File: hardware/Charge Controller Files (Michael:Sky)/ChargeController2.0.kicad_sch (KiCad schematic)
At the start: 90 parts, among them J1 GND_TEST_01x01_Pin, J10 SOL_TEST_01x01_Pin, J13 Conn-1x2, J14 Conn-1x2, J15 Conn-1x2, J17 SCL_MAS_01x01_Pin, J18 SDA_MAS_01x01_Pin, J19 SYS-1x2, J2 SP_01x02_Pin, J3 BATT_TEST_01x01_Pin, J4 3.3V_PULLUP_01x02_Pin, J5 BATT_01x02_Pin, J6 Conn-1x2, J7 Conn-1x2, J8 Conn-1x2, J9 SYS_TEST_01x01_Pin, Q1 SI2318CDS-T1-GE3, Q10 SI2318CDS-T1-GE3, Q11 SI2318CDS-T1-GE3, Q12 SI2318CDS-T1-GE3, Q2 SI2318CDS-T1-GE3, Q3 SI2318CDS-T1-GE3, Q4 SI2318CDS-T1-GE3, Q5 AONS66614, Q6 AONS66614, Q7 AONS66614, Q8 AONS66614, Q9 SI2318CDS-T1-GE3, SW1 100SP1T1B1M1QEH, U1 BQ25756ERRVR

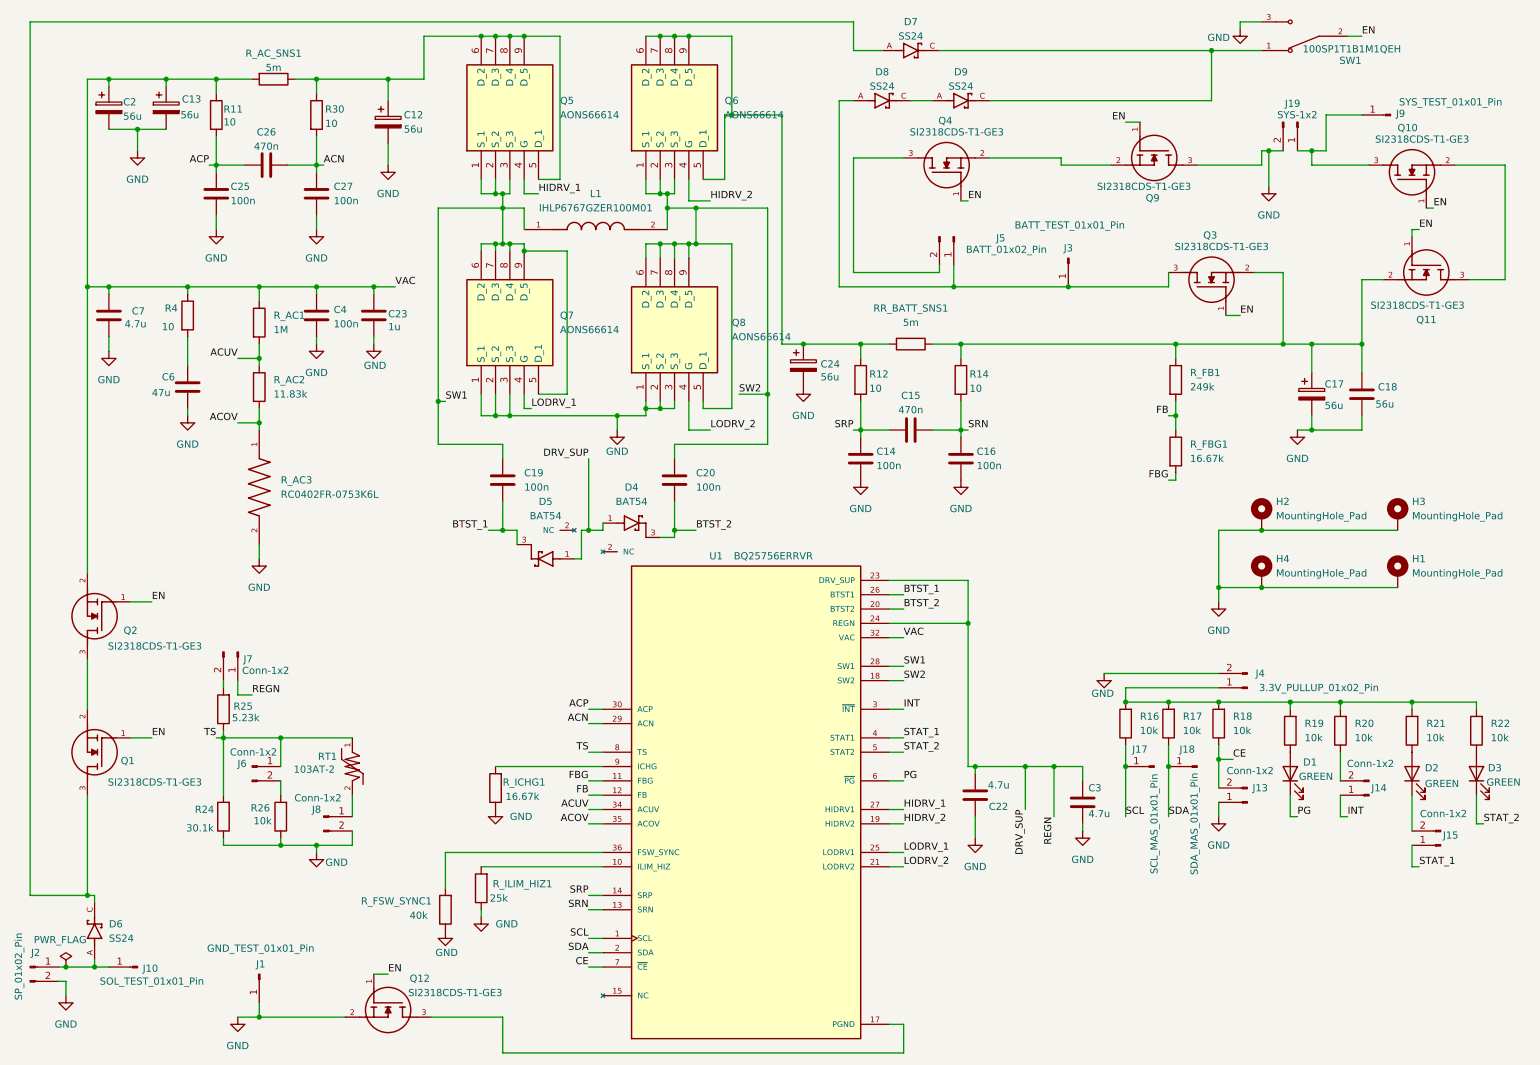
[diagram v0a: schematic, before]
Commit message: Ready for Manufacturing
Final push
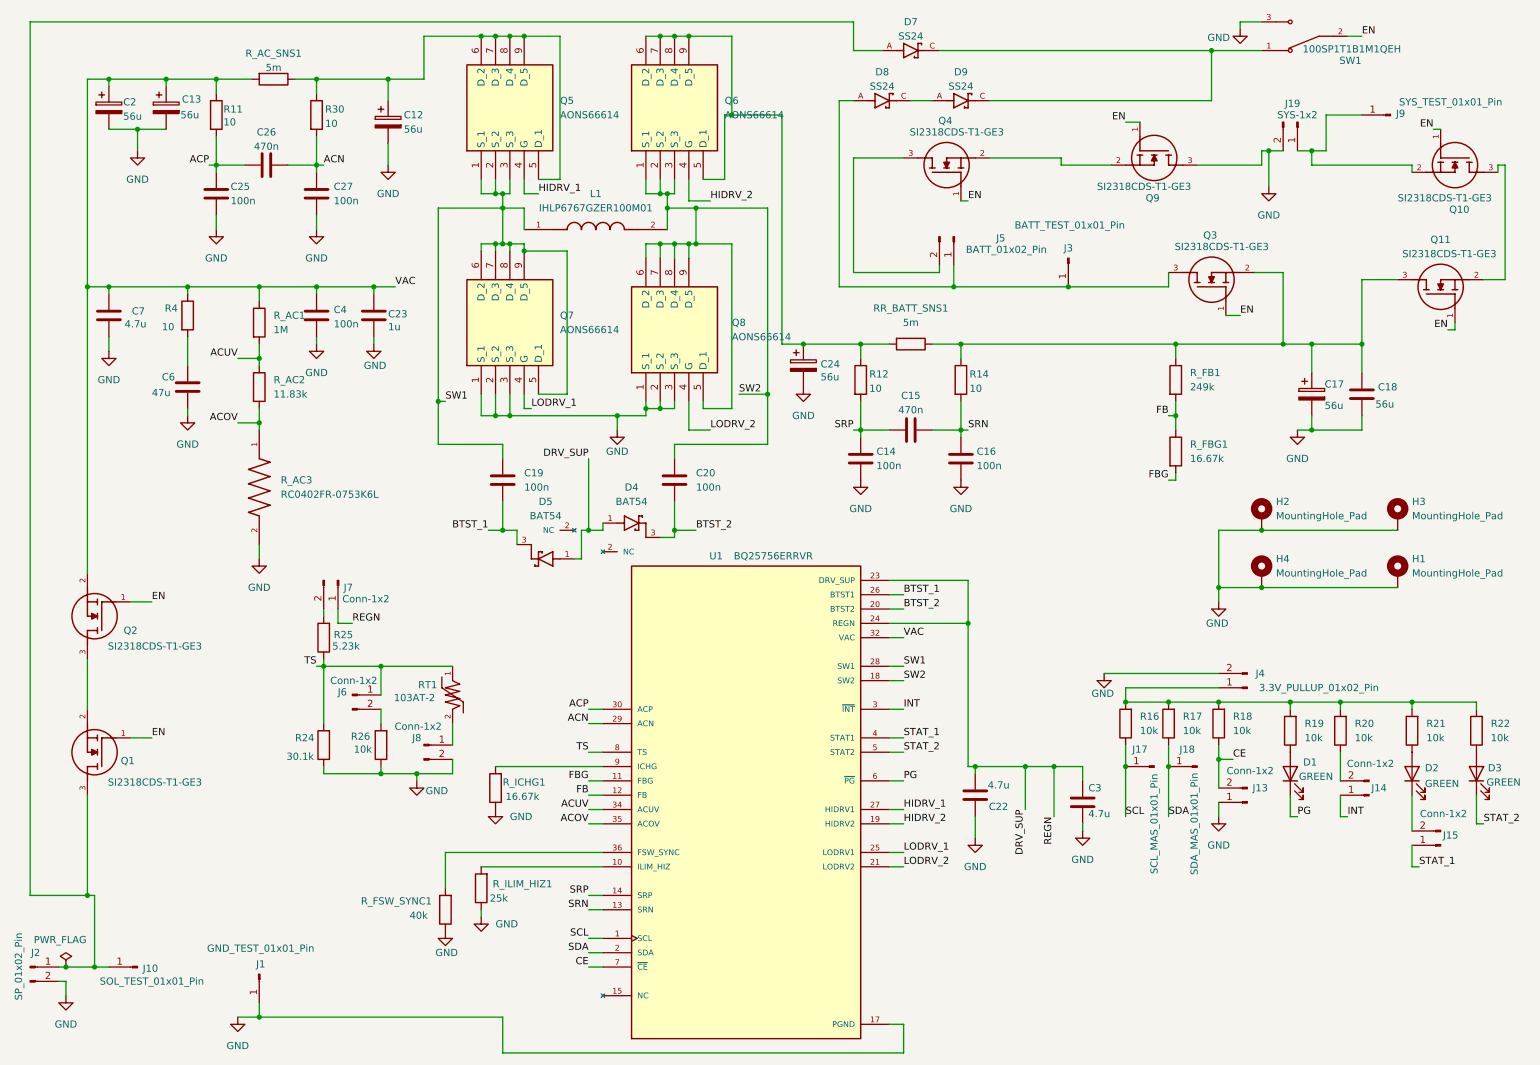
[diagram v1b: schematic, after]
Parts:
- removed D6: SS24, bmsfootprints:SS24, symbol SS24:SS24
- removed Q12: SI2318CDS-T1-GE3, bmsfootprints:SI2318CDS-T1-GE3, symbol SI2318CDS-T1-GE3:SI2318CDS-T1-GE3
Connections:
- net PGND is gone; now on net GND: U1.17 (PGND), U1.22 (PGND), U1.37 (PGND)
- net at C17.1, C18.1, Q3.2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: now also Q11.3; no longer Q11.2
- net at D7.A, Q1.3: now also J10.1 (Pin_1), J2.1 (Pin_1)
- net at J19.1 (Pin_1), J9.1 (Pin_1): now also Q10.2; no longer Q10.3
- new net: Q10.3, Q11.2
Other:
- moved on the sheet: J6, J7, J8, Q10, Q11, R24, R25, R26, RT1
